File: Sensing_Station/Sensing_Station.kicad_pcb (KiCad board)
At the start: 2 copper layers, 50.3 x 66.3 mm, 29 parts, among them J1 Conn_01x02_Pin, J2 Conn_01x02_Pin, J3 Conn_01x02_Pin, Q1 2N7000, Q2 BC550, SW1 ORD 324/10-15 AT, U1 LM35CAZ/NOPB, U2 NE555P, U3 LM358

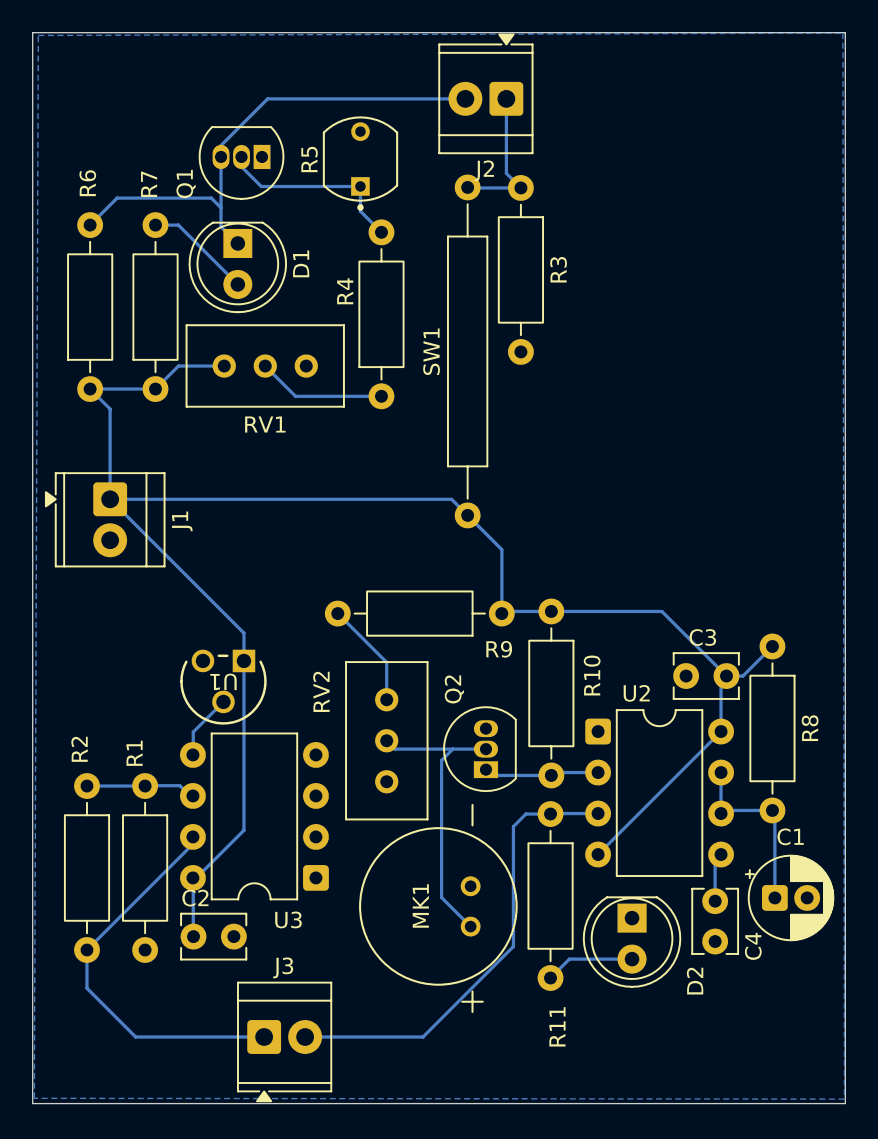
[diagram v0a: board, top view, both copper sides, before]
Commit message: v2.0
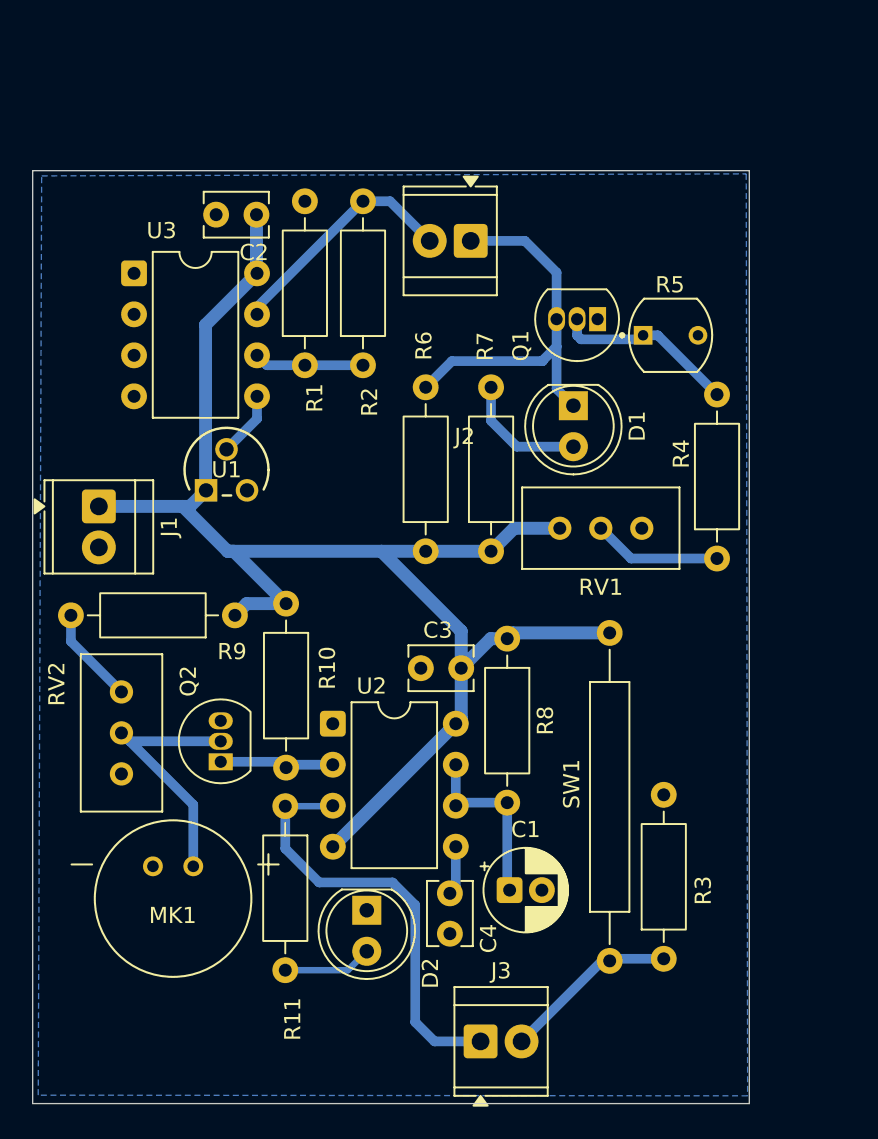
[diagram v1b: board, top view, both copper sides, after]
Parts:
- moved R3 48.6 mm to (118.0, 136.4), turned to 90 degrees
- moved C2 44.9 mm to (92.7, 90.3), turned to 180 degrees
- moved U3 39.1 mm to (85.1, 93.9), turned to 0 degrees
- moved R2 31.2 mm to (99.3, 99.6), turned to 90 degrees
- moved R1 27.9 mm to (95.7, 99.6), turned to 90 degrees
- moved R4 23.1 mm to (121.2, 111.6)
- moved R6 23.1 mm to (103.2, 111.1)
- moved R7 23.1 mm to (107.2, 111.1)
- moved RV1 23.1 mm to (111.5, 109.7)
- moved D1 23.1 mm to (112.3, 102.1)
- moved Q1 23.1 mm to (113.8, 96.8)
- moved R5 22.1 mm to (118.4, 97.8), turned to 0 degrees
- moved R9 16.5 mm to (91.4, 115.1)
- moved C4 16.4 mm to (104.7, 134.8)
- moved D2 16.4 mm to (99.5, 133.4)
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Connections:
- J2 pad 1: /DAQ_MAG -> /DAQ_LIGHT
- J2 pad 2: /DAQ_LIGHT -> /DAQ_TEMP
- J3 pad 1: /DAQ_TEMP -> /DAQ_SOUND
- J3 pad 2: /DAQ_SOUND -> /DAQ_MAG
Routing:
- net +5V: track 111.2 -> 92.8 mm
- net /DAQ_TEMP: track 24.1 -> 14.9 mm
- net /DAQ_LIGHT: track 31.9 -> 24.0 mm
- net Net-(Q2-B): track 18.4 -> 16.5 mm
- net /DAQ_MAG: track 9.21 -> 10.9 mm
- net /DAQ_SOUND: track 28.2 -> 26.9 mm
- net Net-(D1-A): track 6.62 -> 7.84 mm
- net Net-(R9-Pad2): track 6.60 -> 6.04 mm
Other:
- board size 50.3 x 66.3 mm -> 44.4 x 57.8 mm
